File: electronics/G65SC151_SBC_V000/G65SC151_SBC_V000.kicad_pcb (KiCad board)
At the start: 2 copper layers, 90 x 98 mm, 15 parts, among them J14 Conn_01x03, J18 Conn_01x03, J24 Conn_01x03, SW4 switch_DPDT

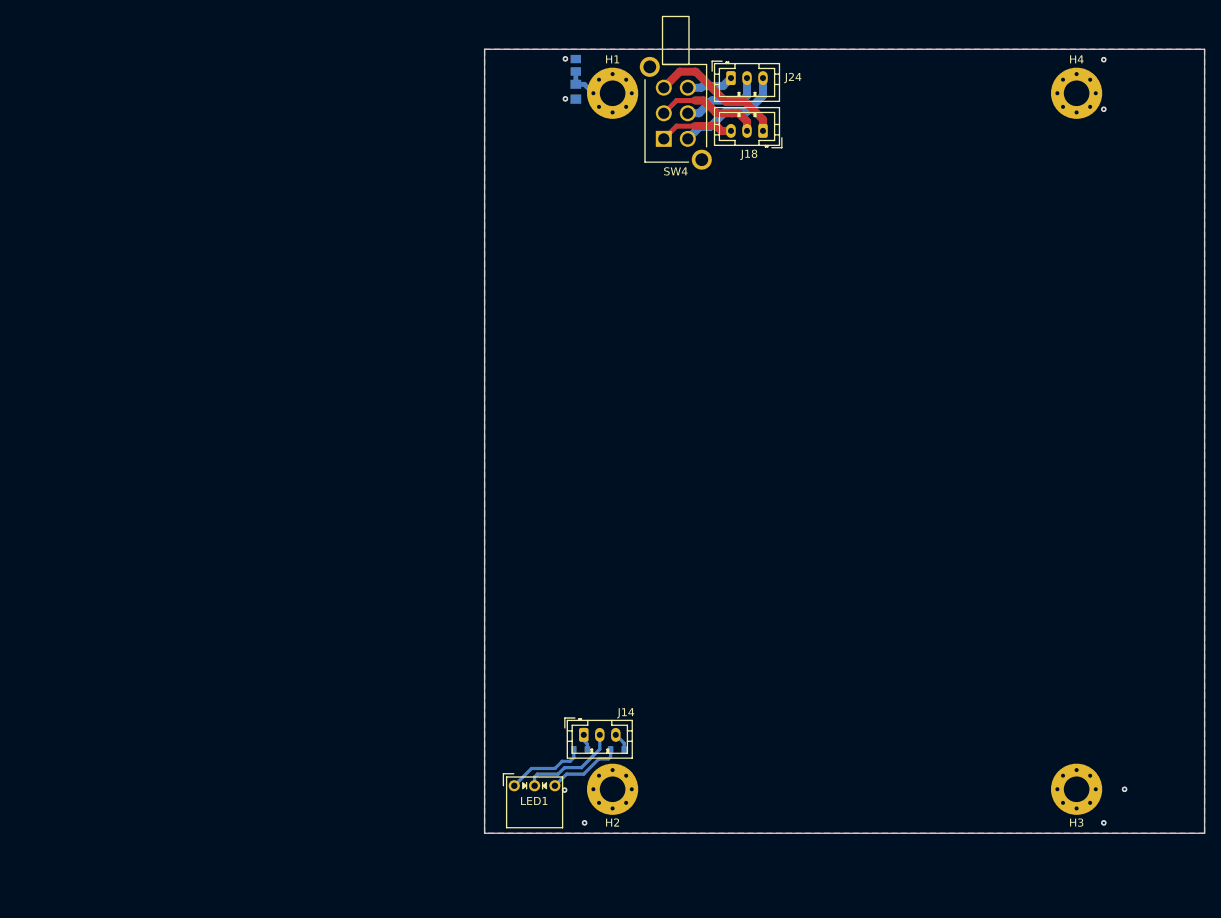
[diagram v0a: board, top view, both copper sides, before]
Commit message: WIP schematic and PCB
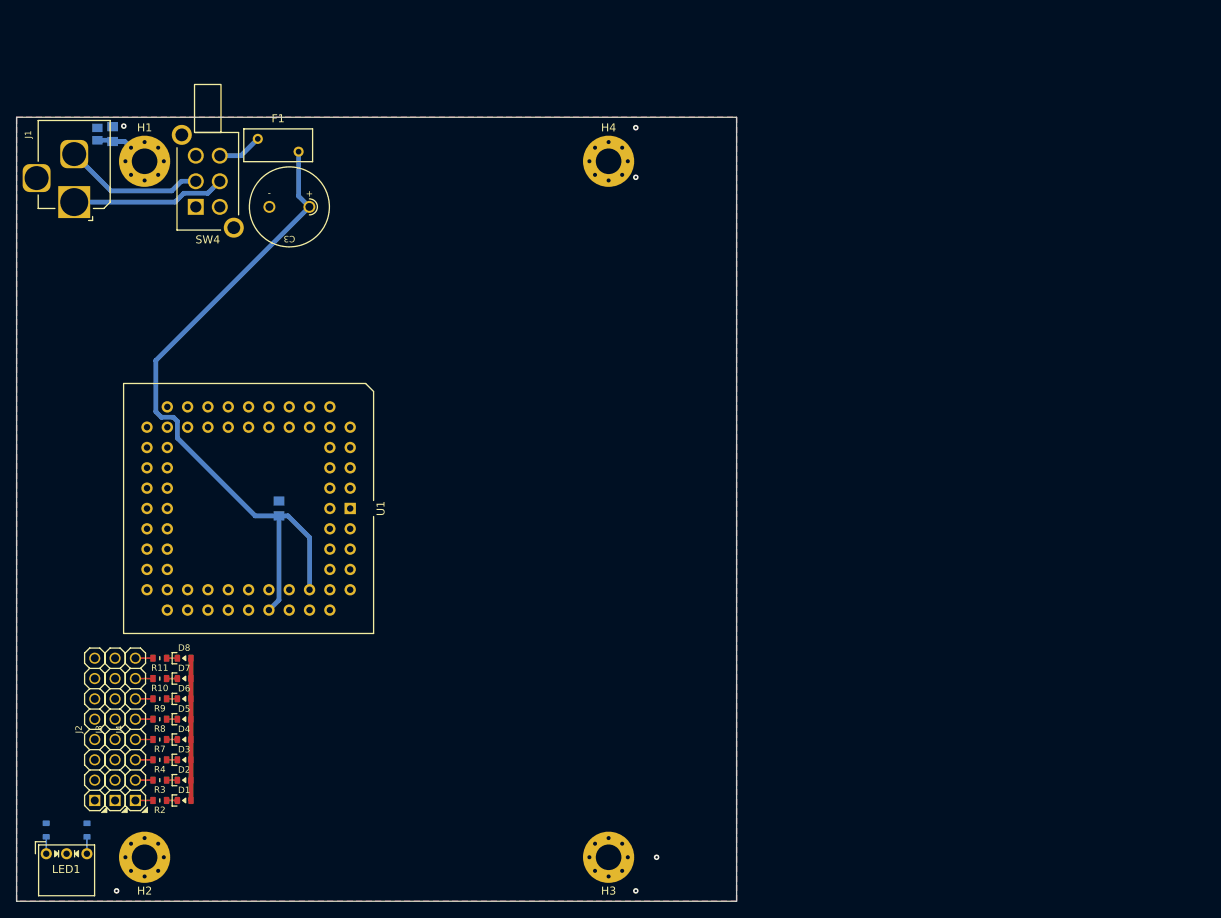
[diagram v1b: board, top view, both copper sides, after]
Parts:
- removed J14, J18, J24: Conn_01x03, Connector_JST:JST_PH_B3B-PH-K_1x03_P2.00mm_Vertical
- added C2: 2.2uF, SquantorRcl:C_0805+0603, B.Cu at (87.8, 99.9)
- added C3: C_Polarized, SquantorCapacitor:C-050-100-elco, F.Cu at (89.1, 62.2)
- added D1: LED, SquantorDiodes:LED_0603_hand, F.Cu at (75.9, 136.4)
- added D2: LED, SquantorDiodes:LED_0603_hand, F.Cu at (75.9, 133.9)
- added D3: LED, SquantorDiodes:LED_0603_hand, F.Cu at (75.9, 131.3)
- added D4: LED, SquantorDiodes:LED_0603_hand, F.Cu at (75.9, 128.8)
- added D5: LED, SquantorDiodes:LED_0603_hand, F.Cu at (75.9, 126.2)
- added D6: LED, SquantorDiodes:LED_0603_hand, F.Cu at (75.9, 123.7)
- added D7: LED, SquantorDiodes:LED_0603_hand, F.Cu at (75.9, 121.2)
- added D8: LED, SquantorDiodes:LED_0603_hand, F.Cu at (75.9, 118.6)
- added F1: Fuse, Fuse:Fuse_BelFuse_0ZRE0012FF_L8.3mm_W3.8mm, F.Cu at (85.2, 53.7)
- added J1: Jack-DC, SquantorConnectors:BarrelJack_Horizontal_Holed, F.Cu at (62.2, 61.6)
- added J2: VSS, SquantorConnectors:Header-0254-1X08-H010, F.Cu at (64.8, 127.5)
- added J3: PORT_A, SquantorConnectors:Header-0254-1X08-H010, F.Cu at (67.3, 127.5)
- added J4: LED, SquantorConnectors:Header-0254-1X08-H010, F.Cu at (69.8, 127.5)
- added R10: 4.7K, SquantorResistor:R_0603_hand, F.Cu at (72.9, 121.2)
- added R11: 4.7K, SquantorResistor:R_0603_hand, F.Cu at (72.9, 118.6)
- added R2: 4.7K, SquantorResistor:R_0603_hand, F.Cu at (72.9, 136.4)
- added R3: 4.7K, SquantorResistor:R_0603_hand, F.Cu at (72.9, 133.9)
- added R4: 4.7K, SquantorResistor:R_0603_hand, F.Cu at (72.9, 131.3)
- added R7: 4.7K, SquantorResistor:R_0603_hand, F.Cu at (72.9, 128.8)
- added R8: 4.7K, SquantorResistor:R_0603_hand, F.Cu at (72.9, 126.2)
- added R9: 4.7K, SquantorResistor:R_0603_hand, F.Cu at (72.9, 123.7)
- added U1: ~, Package_LCC:PLCC-68_THT-Socket, F.Cu at (96.7, 99.9)
- moved R5 67.6 mm to (58.7, 140.1), turned to 90 degrees
- moved R6 67.1 mm to (63.8, 140.1), turned to 90 degrees
- moved R1 60.4 mm to (65.1, 53.1)
- moved H1 59.1 mm to (71.0, 56.5)
- moved H2 59.1 mm to (71.0, 143.5)
- moved H3 59.1 mm to (129.0, 143.5)
- moved H4 59.1 mm to (129.0, 56.5)
- moved LED1 59.1 mm to (61.2, 143.1)
- moved SW4 59.1 mm to (78.9, 59.0)
- moved C1 58.1 mm to (67.0, 53.1), turned to 90 degrees
- moved N1 55.3 mm to (140.7, 143.9)
- moved N2 55.3 mm to (141.7, 147.9)
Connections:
- C1 pad 2: GND -> VSS
- LED1 pad 2: Net-(J14-Pin_2) -> VSS
- R1 pad 2: GND -> VSS
- R5 pad 2: Net-(J14-Pin_1) -> /LED
- R6 pad 2: Net-(J14-Pin_3) -> VDD
- SW4 pad 1: Net-(J18-Pin_3) -> unconnected-(SW4-SW1_P1-Pad1)
- SW4 pad 3: Net-(J18-Pin_1) -> VSS
- SW4 pad 6: Net-(J24-Pin_3) -> unconnected-(SW4-SW2_P2-Pad6)
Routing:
- net VDD: track 0.00 -> 104.6 mm
- net Net-(J18-Pin_1): track 17.1 -> 0.00 mm
- net Net-(J24-Pin_3): track 13.8 -> 0.00 mm
- net Net-(J14-Pin_2): track 12.5 -> 0.00 mm
- net Net-(J18-Pin_3): track 9.31 -> 0.00 mm
- net Net-(SW4-SW2_C1): track 10.5 -> 19.3 mm
- net Net-(LED1-A1): track 9.89 -> 2.11 mm
- net Net-(LED1-A2): track 9.35 -> 2.11 mm
- net Net-(SW4-SW1_C1): track 13.3 -> 17.6 mm
- net Net-(J14-Pin_3): track 2.28 -> 0.00 mm
- net Net-(J4-Pin_8): track 0.00 -> 2.20 mm
- net Net-(J4-Pin_7): track 0.00 -> 2.20 mm
- net Net-(J4-Pin_6): track 0.00 -> 2.20 mm
- net Net-(J4-Pin_5): track 0.00 -> 2.20 mm
- net Net-(J4-Pin_4): track 0.00 -> 2.20 mm
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- added copper zone on B.Cu, net VSS
- added copper zone on F.Cu, net VSS
- removed copper zone on B.Cu, net GND
- removed copper zone on F.Cu, net GND
